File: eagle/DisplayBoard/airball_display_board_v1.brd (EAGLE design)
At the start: 110 x 70 mm, 10 parts, among them J1 MICRO-SD_CARD_SOCKET, J2 USB_A_SMT_FEMALE_NS

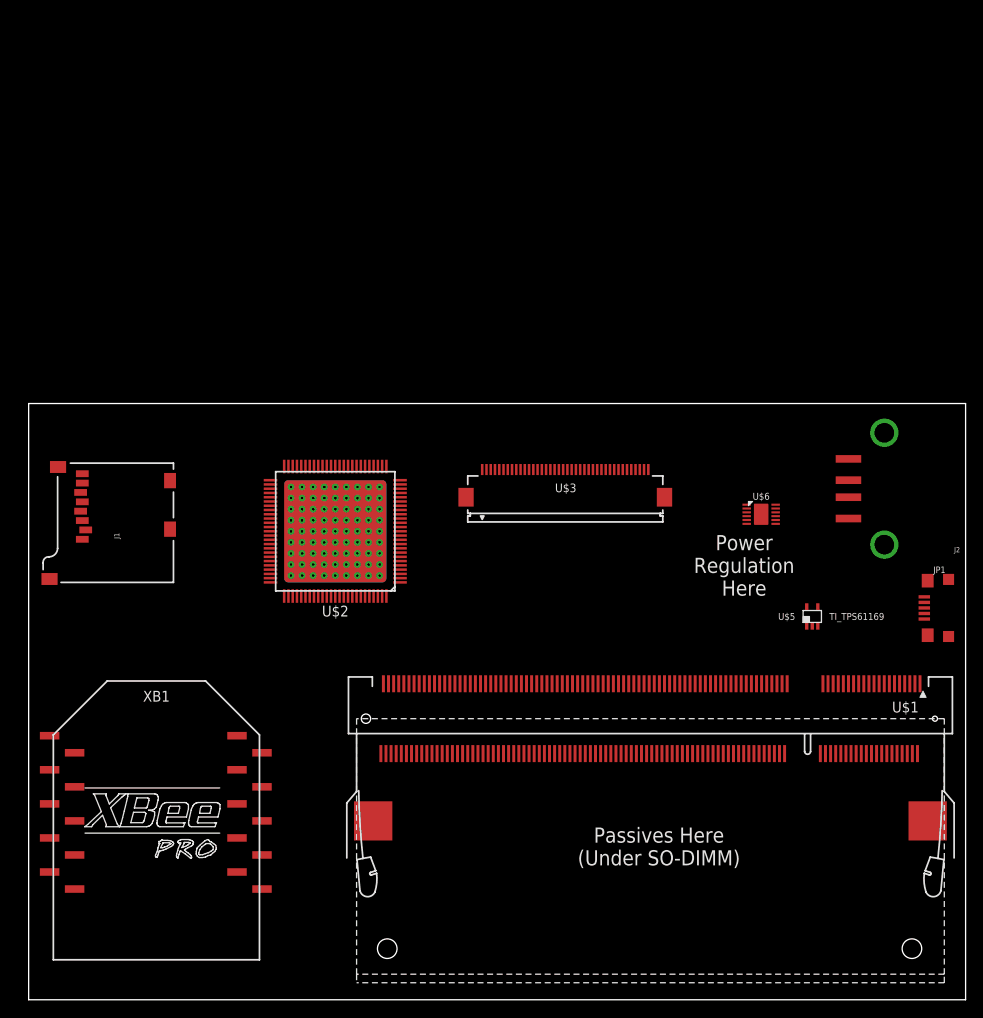
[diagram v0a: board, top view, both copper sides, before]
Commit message: Another WIP commit for display v1
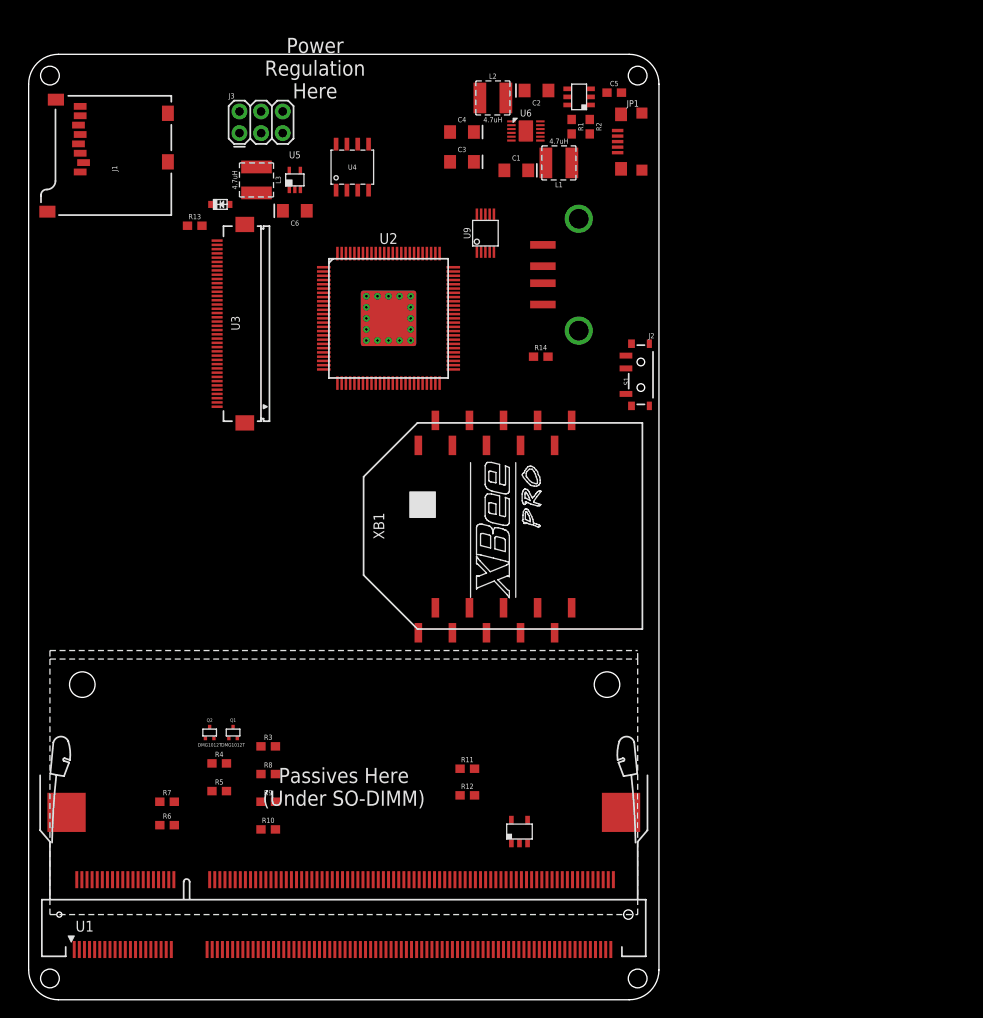
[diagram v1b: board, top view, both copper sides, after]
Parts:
- removed U$1: RPI_CM3-TYCO1376408, airball:RPI_CM_SOCKET
- removed U$2: TFP401, airball:TQFP100_POWER
- removed U$3: TFT_40PIN_FFC, airball:HIROSE_FFC40_FH12-40S-0.5SH
- removed U$5: TI_TPS61169, airball:SOT353-5
- removed U$6: PAM2306, airball:WDFN12
- added C1, C2, C3, C4, C6: 10uF, SparkFun-Capacitors:EIA3216
- added C5: 0.1uF, SparkFun-Capacitors:0603
- added D1: NSR0240H, airball:SOD323
- added J3: AVR_SPI_PROG_3X2PTH, SparkFun-Connectors:2X3
- added L1, L2, L3: 4.7uH, airball:INDUCTOR_SMD_4X4MM
- added Q1, Q2: DMG1012T, airball:SOT523-3
- added R1, R10, R2, R3, R4, R5, R8, R9: 100k, SparkFun-Resistors:0603
- added R11, R12, R6, R7: 4.7k, SparkFun-Resistors:0603
- added R13: 5R1, SparkFun-Resistors:0603
- added R14: 10k, SparkFun-Resistors:0603
- added S1: (no value), SparkFun-Switches:SWITCH_SPST_SMD_A
- added U1: RPI_CM3-TYCO1376408, airball:RPI_CM_SOCKET
- added U2: TFP401A, airball:TQFP100_POWER_LITE
- added U3: TFT_40PIN_FFC-TOP, airball:HIROSE_FFC40_FH12-40S-0.5SH
- added U4: ATtiny85, airball:SOIC8
- added U5: TPS61169, airball:SOT353-5
- added U6: PAM2306AYPKE, airball:WDFN12
- added U7: LM3880MF-1AB, airball:SOT23-6
- added U8: 24LC02B, airball:SOT23-5
- added U9: FSUSB42, airball:MSOP10
- J1: value MICRO-SD_CARD_SOCKET -> (none); device SparkFun-Connectors:MICRO-SD-SOCKET -> airball:MICRO-SD-SOCKET
- moved JP1 65.5 mm to (72.0, 100.8)
- moved XB1 52.1 mm to (54.8, 55.6), turned to 90 degrees
- moved J2 43.8 mm to (67.1, 85.1)
- moved J1 43.1 mm to (16.8, 106.1)
- moved U$4 27.3 mm to (37.0, 55.5), turned to 270 degrees
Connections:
- removed net AGND: U$2.79, U$2.83, U$2.87, U$2.89, U$2.92
- removed net AVDD: U$2.82, U$2.84, U$2.88, U$2.95
- removed net DGND: U$2.39, U$2.5, U$2.68
- removed net DVDD: U$2.38, U$2.6, U$2.67
- removed net LED_A: U$3.2
- removed net LED_K: U$3.1
- removed net N$27: U$2.27, U$3.20
- removed net N$28: U$2.10, U$3.21
- removed net N$29: U$2.11, U$3.22
- removed net N$30: U$2.12, U$3.23
- removed net N$31: U$2.13, U$3.24
- removed net N$32: U$2.14, U$3.25
- removed net N$33: U$2.15, U$3.26
- removed net N$34: U$2.16, U$3.27
- removed net N$35: U$2.17, U$3.28
- removed net N$36: U$2.46, U$3.34
- removed net N$37: U$2.44, U$3.30
- removed net N$38: U$2.48, U$3.32
- removed net N$39: U$2.47, U$3.33
- removed net N$40: U$2.8, U$3.31
- removed net OGND: U$2.19, U$2.28, U$2.45, U$2.58, U$2.76
- removed net OVDD: U$2.18, U$2.29, U$2.43, U$2.57, U$2.78
- removed net PGND: U$2.98
- removed net PVDD: U$2.97
- removed net SW: U$5.1
- removed net THERMAL: U$2.TH1, U$2.TH10, U$2.TH11, U$2.TH12, U$2.TH13, U$2.TH14, U$2.TH15, U$2.TH16, U$2.TH17, U$2.TH18, U$2.TH19, U$2.TH2, U$2.TH20, U$2.TH21, U$2.TH22, U$2.TH23, U$2.TH24, U$2.TH25, U$2.TH26, U$2.TH27, U$2.TH28, U$2.TH29, U$2.TH3, U$2.TH30, U$2.TH31, U$2.TH32, U$2.TH33, U$2.TH34, U$2.TH35, U$2.TH36, U$2.TH37, U$2.TH38, U$2.TH39, U$2.TH4, U$2.TH40, U$2.TH41, U$2.TH42, U$2.TH43, U$2.TH44, U$2.TH45, U$2.TH46, U$2.TH47, U$2.TH48, U$2.TH49, U$2.TH5, U$2.TH50, U$2.TH51, U$2.TH52, U$2.TH53, U$2.TH54, U$2.TH55, U$2.TH56, U$2.TH57, U$2.TH58, U$2.TH59, U$2.TH6, U$2.TH60, U$2.TH61, U$2.TH62, U$2.TH63, U$2.TH64, U$2.TH65, U$2.TH66, U$2.TH67, U$2.TH68, U$2.TH69, U$2.TH7, U$2.TH70, U$2.TH71, U$2.TH72, U$2.TH73, U$2.TH74, U$2.TH75, U$2.TH76, U$2.TH77, U$2.TH78, U$2.TH79, U$2.TH8, U$2.TH80, U$2.TH81, U$2.TH9, U$2.THA, U$2.THB
- removed net VBAT: U$1.197, U$1.198, U$1.199, U$1.200
- removed net VBUS: J2.VBUS
- removed net VCC: XB1.1
- removed net VDAC: U$1.189, U$1.190
- removed net VDD: U$3.4
- removed net VDD_GPIO0_27: U$1.39, U$1.40
- removed net VDD_GPIO28_45: U$1.41, U$1.42
- removed net VDD_SDX: U$1.4, U$1.6
- removed net VIN: U$5.5
- new net B0: U2.10, U3.20
- new net B1: U2.11, U3.19
- new net B2: U2.12, U3.18
- new net B3: U2.13, U3.17
- new net B4: U2.14, U3.16
- new net B5: U2.15, U3.15
- new net B6: U2.16, U3.14
- new net B7: U2.17, U3.13
- new net BKL_LED_A: C6.+, D1.K, U3.39
- new net BKL_LED_K: R13.2, U3.40, U5.3
- new net BKL_MISO: J3.1, U4.6
- new net BKL_MOSI: J3.4, R7.2, U4.5
- new net BKL_RST: J3.5, U4.1
- new net BKL_SCK: J3.3, R6.2, U4.7
- new net DE: U2.46, U3.7
- new net EMMC_DISABLE: Q1.2, U1.2
- new net EMMC_EN: Q2.1, R5.1, U1.90
- new net EN_1V8: R2.1, U6.12, U7.5
- new net EN_3V3: R1.1, U6.6, U7.6
- new net G0: U2.20, U3.28
- new net G1: U2.21, U3.27
- new net G2: U2.22, U3.26
- new net G3: U2.23, U3.25
- new net G4: U2.24, U3.24
- new net G5: U2.25, U3.23
- new net G6: U2.26, U3.22
- new net G7: U2.27, U3.21
- new net HDMI_EDID_SCL: U1.175, U8.1
- new net HDMI_EDID_SDA: U1.173, U8.3
- new net HSYNC: U2.48, U3.9
- new net LED_ACT: Q1.3, Q2.2
- new net PCLK: U2.44, U3.11
- new net R0: U2.30, U3.36
- new net R1: U2.31, U3.35
- new net R2: U2.32, U3.34
- new net R3: U2.33, U3.33
- new net R4: U2.34, U3.32
- new net R5: U2.35, U3.31
- new net R6: U2.36, U3.30
- new net R7: U2.37, U3.29
- new net RXD0: U1.53, XB1.2
- new net SCDT: U2.8, U3.10
- new net SCL1: R12.2, R6.1, U1.11
- new net SDA1: R11.2, R7.1, U1.9
- new net TXD0: U1.51, XB1.3
- new net USB_A_N: J2.D-, U9.6
- new net USB_A_P: J2.D+, U9.7
- new net USB_BOOT_EN: Q1.1, R4.2
- new net USB_B_N: JP1.2, U9.8
- new net USB_B_P: JP1.3, U9.9
- new net USB_N: U1.167, U9.4
- new net USB_P: U1.165, U9.3
- new net VCC_5V0: C3.+, C4.+, J2.VBUS, J3.2, JP1.1, L3.1, R1.2, R2.2, U1.197, U1.198, U1.199, U1.200, U4.8, U5.5, U6.1, U6.7, U7.1
- new net VSYNC: U2.47, U3.8
- net GND: now also C1.-, C2.-, C3.-, C4.-, C5.2, C6.-, J1.6, J1.SH@1, J1.SH@2, J2.SHLD1, J2.SHLD2, J3.6, JP1.5, JP1.SH@1, JP1.SH@2, JP1.SH@3, JP1.SH@4, Q2.3, R10.1, R13.1, R3.1, R4.1, R8.1, R9.1, S1.3, U1.1, U1.103, U1.104, U1.109, U1.110, U1.115, U1.116, U1.121, U1.122, U1.127, U1.13, U1.133, U1.134, U1.139, U1.14, U1.140, U1.145, U1.146, U1.151, U1.152, U1.157, U1.163, U1.164, U1.168, U1.169, U1.170, U1.181, U1.182, U1.187, U1.188, U1.19, U1.195, U1.196, U1.20, U1.25, U1.26, U1.31, U1.32, U1.37, U1.38, U1.43, U1.44, U1.49, U1.50, U1.55, U1.56, U1.61, U1.62, U1.67, U1.68, U1.7, U1.73, U1.74, U1.79, U1.8, U1.80, U1.85, U1.86, U1.91, U1.92, U1.97, U1.98, U2.1, U2.100, U2.19, U2.28, U2.39, U2.4, U2.45, U2.5, U2.58, U2.68, U2.76, U2.79, U2.83, U2.87, U2.89, U2.92, U2.98, U2.TH21, U2.TH22, U2.TH23, U2.TH24, U2.TH25, U2.TH30, U2.TH34, U2.TH39, U2.TH43, U2.TH48, U2.TH52, U2.TH57, U2.TH58, U2.TH59, U2.TH60, U2.TH61, U2.THA, U2.THB, U3.12, U3.38, U3.5, U4.4, U5.2, U6.3, U6.9, U7.2, U8.2, U8.5, U9.10, U9.5; no longer U$1.1, U$1.103, U$1.104, U$1.109, U$1.110, U$1.115, U$1.116, U$1.121, U$1.122, U$1.127, U$1.13, U$1.133, U$1.134, U$1.139, U$1.14, U$1.140, U$1.145, U$1.146, U$1.151, U$1.152, U$1.157, U$1.163, U$1.164, U$1.169, U$1.170, U$1.181, U$1.182, U$1.187, U$1.188, U$1.19, U$1.195, U$1.196, U$1.20, U$1.25, U$1.26, U$1.31, U$1.32, U$1.37, U$1.38, U$1.43, U$1.44, U$1.49, U$1.50, U$1.55, U$1.56, U$1.61, U$1.62, U$1.67, U$1.68, U$1.7, U$1.73, U$1.74, U$1.79, U$1.8, U$1.80, U$1.85, U$1.86, U$1.91, U$1.92, U$1.97, U$1.98, U$3.29, U$3.3, U$3.36, U$5.2
- net N$1: now also J1.5, U1.10; no longer J1.SCLK, U$1.10
- net N$10: now also U1.113, U2.93; no longer U$1.113, U$2.93
- net N$11: now also U1.111, U2.94; no longer U$1.111, U$2.94
- net N$12: now also J1.8, U1.18; no longer U$2.30, U$3.5
- net N$13: now also J1.1, U1.22; no longer U$2.31, U$3.6
- net N$14: now also J1.2, U1.24; no longer U$2.32, U$3.7
- net N$15: now also L1.1, U6.8; no longer U$2.33, U$3.8
- net N$16: now also L2.1, U6.2; no longer U$2.34, U$3.9
- net N$17: now also C5.1, U7.3; no longer U$2.35, U$3.10
- net N$18: now also R3.2, U1.30; no longer U$2.36, U$3.11
- net N$19: now also XB1.13; no longer U$2.37, U$3.12
- net N$2: now also J1.3, U1.12; no longer J1.DI, U$1.16
- net N$20: now also XB1.15; no longer U$2.20, U$3.13
- net N$21: now also R8.2, U1.28; no longer U$2.21, U$3.14
- net N$22: now also U4.3, U5.4; no longer U$2.22, U$3.15
- net N$23: now also R9.2, U1.84; no longer U$2.23, U$3.16
- net N$24: now also R10.2, U1.82; no longer U$2.24, U$3.17
- net N$25: now also D1.A, L3.2, U5.1; no longer U$2.25, U$3.18
- net N$26: now also R14.2, S1.2, U9.2; no longer U$2.26, U$3.19
- net N$3: now also J1.7, U1.16; no longer J1.DO, U$1.18
- net N$4: now also U1.131, U2.80; no longer U$1.131, U$2.80
- net N$5: now also U1.129, U2.81; no longer U$1.129, U$2.81
- net N$6: now also U1.125, U2.85; no longer U$1.125, U$2.85
- net N$7: now also U1.123, U2.86; no longer U$1.123, U$2.86
- net N$8: now also U1.119, U2.90; no longer U$1.119, U$2.90
- net N$9: now also U1.117, U2.91; no longer U$1.117, U$2.91
- net VCC_1V8: now also C2.+, L2.2, R5.2, U1.183, U1.184, U1.185, U1.186, U6.10; no longer U$1.183, U$1.184, U$1.185, U$1.186
- net VCC_3V3: now also C1.+, J1.4, L1.2, R11.1, R12.1, R14.1, U1.189, U1.190, U1.191, U1.192, U1.193, U1.194, U1.39, U1.4, U1.40, U1.41, U1.42, U1.6, U2.18, U2.29, U2.3, U2.38, U2.43, U2.57, U2.6, U2.67, U2.7, U2.78, U2.82, U2.84, U2.88, U2.95, U2.97, U2.99, U3.37, U6.4, U8.4, U9.1, XB1.1; no longer U$1.191, U$1.192, U$1.193, U$1.194
- net VDD_CORE: now also U1.179; no longer U$1.179
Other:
- board size 110 x 70 mm -> 74 x 111 mm

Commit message: Airball Display Board v1 as built
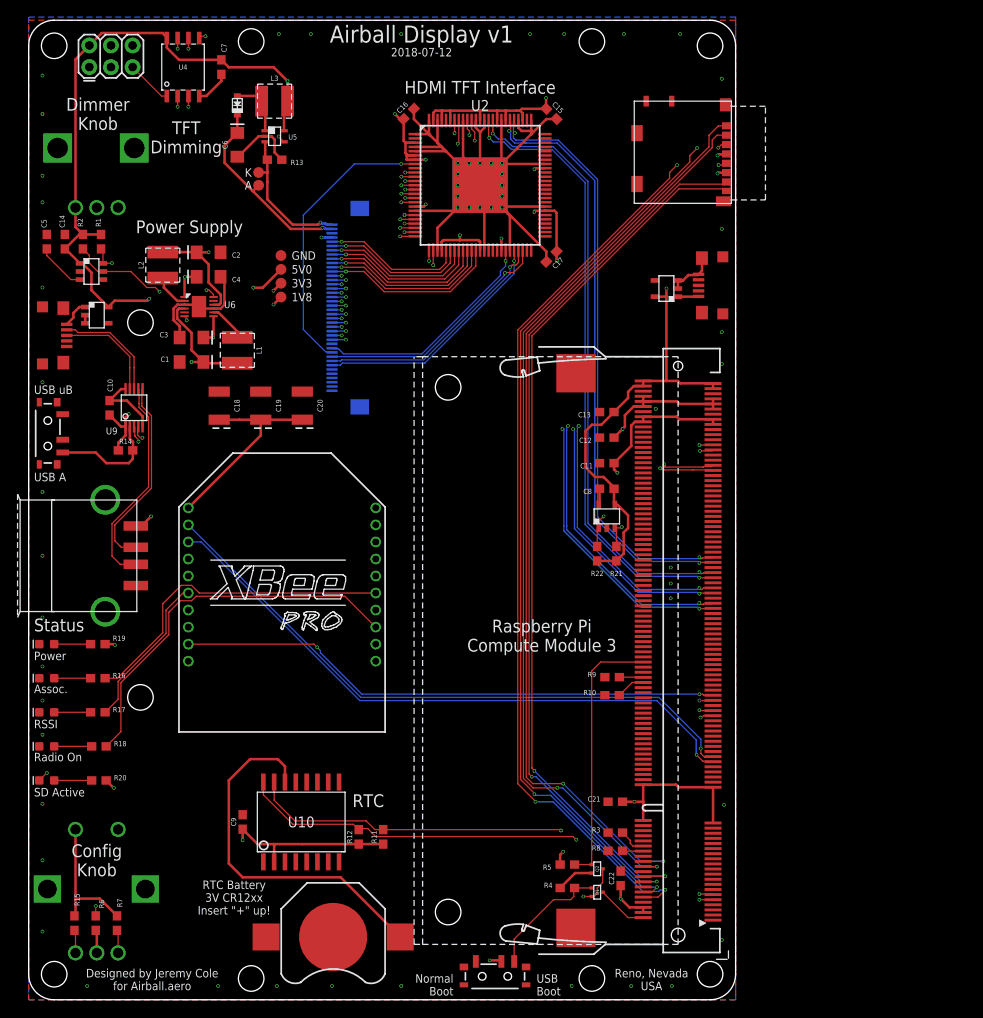
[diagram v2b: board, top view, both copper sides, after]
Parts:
- removed J2: USB_A_SMT_FEMALE_NS, SparkFun-Connectors:USB-A-S-NOSILK-FEMALE
- removed JP1: USB_MICROB_PLUG, airball:USB_MICRO_B_TYCO
- added BT1: (no value), SparkFun-Batteries:BATTCON_12MM
- added C10, C11, C12, C13, C14, C15, C16, C17, C21, C22, C7, C8, C9: 0.1uF, SparkFun-Capacitors:0603
- added C18, C19, C20: 47uF, SparkFun-Capacitors:EIA3528
- added D2, D3, D4, D5, D6: (no value), SparkFun-LED:LED-0603
- added R15, R21, R22: 4.7k, SparkFun-Resistors:0603
- added R16, R17, R18, R19, R20: 330, SparkFun-Resistors:0603
- added S2: (no value), SparkFun-Switches:SWITCH_SPST_SMD_A
- added TP_1V8, TP_3V3, TP_5V0, TP_BKL_LED_A, TP_BKL_LED_K, TP_GND: (no value), SparkFun-Connectors:PAD.03X.05
- added U$1: (no value), airball:BOURNS_PEC11L
- added U10: DS3231, airball:SOIC16W
- added U11, U12: (no value), airball:SOT23-5
- added USB_A: USB_A, airball:FCI_USB_A_87583
- added USB_B_1, USB_B_2: USB_MICROB_PLUG, airball:USB_MICRO_B_TYCO
- added VR1: 10k, airball:BOURNS_PTV09A
- J1: device airball:MICRO-SD-SOCKET -> airball:MOLEX_MICRO_SD_104031
- U1: value RPI_CM3-TYCO1376408 -> RPI_CM3-AMP_1473149; device airball:RPI_CM_SOCKET -> airball:AMP_1473149
- U3: value TFT_40PIN_FFC-TOP -> TFT_40PIN_FFC-BOT
- U4: device airball:SOIC8 -> airball:SOIC8-5.4
- XB1: value XBEE-PRO-SMD -> XBEE-PRO; device airball:XBEE-PRO-SMD -> airball:XBEE-PRO
- moved S1 70.0 mm to (2.25, 66.5), turned to 90 degrees
- moved C5 68.9 mm to (2.12, 89.0), turned to 90 degrees
- moved J1 66.1 mm to (82.5, 99.5)
- moved R2 61.0 mm to (6.38, 89.0), turned to 90 degrees
- moved U7 60.8 mm to (7.38, 85.5), turned to 270 degrees
- moved R1 56.9 mm to (8.50, 89.0), turned to 90 degrees
- moved U1 50.0 mm to (76.2, 41.0), turned to 90 degrees
- moved R14 50.0 mm to (11.4, 64.5)
- moved Q2 48.2 mm to (66.8, 15.4), turned to 270 degrees
- moved Q1 46.7 mm to (66.8, 12.6), turned to 270 degrees
- moved U9 46.1 mm to (12.4, 69.5)
- moved C1 44.3 mm to (19.1, 74.9)
- moved L1 43.7 mm to (24.5, 76.2), turned to 270 degrees
- moved U6 43.6 mm to (20.0, 81.4)
- moved L2 43.4 mm to (15.8, 86.2), turned to 90 degrees
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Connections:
- net N$1 renamed SD_CLK
- net N$10 renamed HDMI_CLK_P
- net N$11 renamed HDMI_CLK_N
- net N$12 renamed SD_D1
- net N$13 renamed SD_D2
- net N$14 renamed SD_D3
- net N$15 renamed L_VCC_3V3
- net N$16 renamed L_VCC_1V8
- net N$18 renamed PD_GPIO29
- net N$2 renamed SD_CMD
- net N$21 renamed PD_GPIO28
- net N$22 renamed BKL_PWM
- net N$23 renamed PD_GPIO45
- net N$24 renamed PD_GPIO44
- net N$25 renamed L_BKL
- net N$3 renamed SD_D0
- net N$4 renamed HDMI_D2_P
- net N$5 renamed HDMI_D2_N
- net N$6 renamed HDMI_D1_P
- net N$7 renamed HDMI_D1_N
- net N$8 renamed HDMI_D0_P
- net N$9 renamed HDMI_D0_N
- removed net N$19: XB1.13
- removed net N$20: XB1.15
- removed net VDD_CORE: U1.179
- new net BKL_ADJ: U4.2, VR1.2
- new net ENC_A: R7.2, U$1.A, U1.69
- new net ENC_B: R15.2, U$1.B, U1.71
- new net ENC_SW: R6.2, U$1.1, U1.75
- new net RTC_VBAT: BT1.PWR@1, U10.14
- new net R_POWER: D5.A, R19.1
- new net R_SD_ACT: D6.A, R20.1
- new net R_XBEE_ASSOC: D2.A, R16.1
- new net R_XBEE_ON: D4.A, R18.1
- new net R_XBEE_RSSI: D3.A, R17.1
- new net USB_A_VCC: U12.1, USB_B_1.1
- new net USB_B_VCC: U11.1, USB_B_2.1
- new net XBEE_ASSOC: R16.2, XB1.15
- new net XBEE_ON: R18.2, XB1.13
- new net XBEE_RSSI: R17.2, XB1.6
- new net XBEE_SLEEP_RQ: U1.77, XB1.9
- net B0: now also U3.21; no longer U3.20
- net B1: now also U3.22; no longer U3.19
- net B2: now also U3.23; no longer U3.18
- net B3: now also U3.24; no longer U3.17
- net B4: now also U3.25; no longer U3.16
- net B5: now also U3.26; no longer U3.15
- net B6: now also U3.27; no longer U3.14
- net B7: now also U3.28; no longer U3.13
- net BKL_LED_A: now also TP_BKL_LED_A.P$1, U3.2; no longer U3.39
- net BKL_LED_K: now also TP_BKL_LED_K.P$1, U3.1; no longer U3.40
- net BKL_MOSI: no longer R7.2
- net BKL_SCK: no longer R6.2
- net DE: now also U3.34; no longer U3.7
- net G0: now also U3.13; no longer U3.28
- net G1: now also U3.14; no longer U3.27
- net G2: now also U3.15; no longer U3.26
- net G3: now also U3.16; no longer U3.25
- net G4: now also U3.17; no longer U3.24
- net G5: now also U3.18; no longer U3.23
- net G6: now also U3.19; no longer U3.22
- net G7: now also U3.20; no longer U3.21
- net GND: now also BT1.GND, C10.1, C11.2, C12.2, C13.2, C14.2, C15.2, C16.2, C17.2, C18.C, C19.C, C20.C, C21.2, C22.2, C7.2, C8.2, C9.2, D2.C, D3.C, D4.C, D5.C, J1.CD1, J1.CD2, J1.SH@3, J1.SH@4, R6.1, S1.2, TP_GND.P$1, U$1.C, U10.10, U10.11, U10.12, U10.13, U10.5, U10.6, U10.7, U10.8, U10.9, U11.2, U11.3, U12.2, U12.3, U3.29, U3.3, U3.36, U6.TH, USB_A.GND, USB_A.SH@1, USB_A.SH@2, USB_B_1.5, USB_B_1.SH@1, USB_B_1.SH@2, USB_B_1.SH@3, USB_B_1.SH@4, USB_B_2.5, USB_B_2.SH@1, USB_B_2.SH@2, USB_B_2.SH@3, USB_B_2.SH@4, VR1.1; no longer J2.GND, J2.SHLD1, J2.SHLD2, JP1.5, JP1.SH@1, JP1.SH@2, JP1.SH@3, JP1.SH@4, S1.3, U3.12, U3.38, U3.5
- net HDMI_EDID_SCL: now also R22.1
- net HDMI_EDID_SDA: now also R21.1
- net HSYNC: now also U3.32; no longer U3.9
- net LED_ACT: now also D6.C
- net N$26: now also S1.1; no longer S1.2
- net PCLK: now also U3.30; no longer U3.11
- net R0: now also U3.5; no longer U3.36
- net R1: now also U3.6; no longer U3.35
- net R2: now also U3.7; no longer U3.34
- net R3: now also U3.8; no longer U3.33
- net R4: now also U3.9; no longer U3.32
- net R5: now also U3.10; no longer U3.31
- net R6: now also U3.11; no longer U3.30
- net R7: now also U3.12; no longer U3.29
- net SCDT: now also U3.31; no longer U3.10
- net SCL1: now also U10.16; no longer R6.1
- net SDA1: now also U10.15; no longer R7.1
- net USB_A_N: now also USB_A.D-; no longer J2.D-
- net USB_A_P: now also USB_A.D+; no longer J2.D+
- net USB_BOOT_EN: now also S2.1
- net USB_B_N: now also USB_B_1.2; no longer JP1.2
- net USB_B_P: now also USB_B_1.3; no longer JP1.3
- net VCC_1V8: now also C11.1, S2.2, TP_1V8.P$1
- net VCC_3V3: now also C10.2, C12.1, C15.1, C16.1, C17.1, C18.A, C19.A, C20.A, C21.1, C22.1, C9.1, R15.1, R20.2, R7.1, TP_3V3.P$1, U$1.2, U10.2, U3.4; no longer U3.37, U8.4
- net VCC_5V0: now also C13.1, C14.1, C7.1, C8.1, R19.2, R21.2, R22.2, TP_5V0.P$1, U11.5, U12.5, U8.4, USB_A.VBUS, VR1.3; no longer J2.VBUS, JP1.1
- net VSYNC: now also U3.33; no longer U3.8
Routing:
- net VCC_5V0: track 0.00 -> 268.4 mm, vias 0 -> 8
- net VCC_3V3: track 0.00 -> 179.8 mm, vias 0 -> 19
- net GND: track 0.00 -> 143.9 mm, vias 0 -> 41
- net SD_CLK: track 0.00 -> 111.9 mm, vias 0 -> 4
- net SD_CMD: track 0.00 -> 109.5 mm, vias 0 -> 4
- net SD_D2: track 0.00 -> 108.6 mm, vias 0 -> 2
- net SD_D3: track 0.00 -> 108.3 mm, vias 0 -> 2
- net SD_D1: track 0.00 -> 104.4 mm, vias 0 -> 2
- net SD_D0: track 0.00 -> 104.0 mm, vias 0 -> 2
- net ENC_SW: track 0.00 -> 98.4 mm, vias 0 -> 2
- net ENC_B: track 0.00 -> 89.4 mm, vias 0 -> 1
- net ENC_A: track 0.00 -> 84.3 mm, vias 0 -> 1
- net HDMI_CLK_N: track 0.00 -> 81.4 mm, vias 0 -> 3
- net HDMI_CLK_P: track 0.00 -> 81.0 mm, vias 0 -> 3
- net HDMI_D0_N: track 0.00 -> 78.6 mm, vias 0 -> 3
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- added copper zone on layer 1, net GND
- added copper zone on layer 16, net GND
- added copper zone on layer 15, net VCC_1V8
- added copper zone on layer 2, net VCC_3V3
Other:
- board size 74 x 111 mm -> 83 x 115 mm
- board text added: "1V8"
- board text added: "2018-07-12"
- board text added: "3V3"
- board text added: "5V0"
- board text added: "A"
- board text added: "Airball Display v1"
- board text added: "Assoc."
- board text added: "Config Knob"
- board text added: "Designed by Jeremy Cole for Airball.aero"
- board text added: "Dimmer Knob"
- board text added: "GND"
- board text added: "HDMI TFT Interface"
- board text added: "K"
- board text added: "Normal Boot"
- board text added: "Power"
- board text added: "Power Supply"
- board text added: "RSSI"
- board text added: "RTC"
- board text added: "RTC Battery 3V CR12xx Insert "+" up!"
- board text added: "Radio On"
- board text added: "Raspberry Pi Compute Module 3"
- board text added: "Reno, Nevada USA"
- board text added: "SD Active"
- board text added: "Status"
- board text added: "TFT Dimming"
- board text added: "USB A"
- board text added: "USB Boot"
- board text added: "USB uB"
- board text removed: "Passives Here (Under SO-DIMM)"
- board text removed: "Power Regulation Here"
